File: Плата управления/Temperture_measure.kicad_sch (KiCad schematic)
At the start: 3 parts

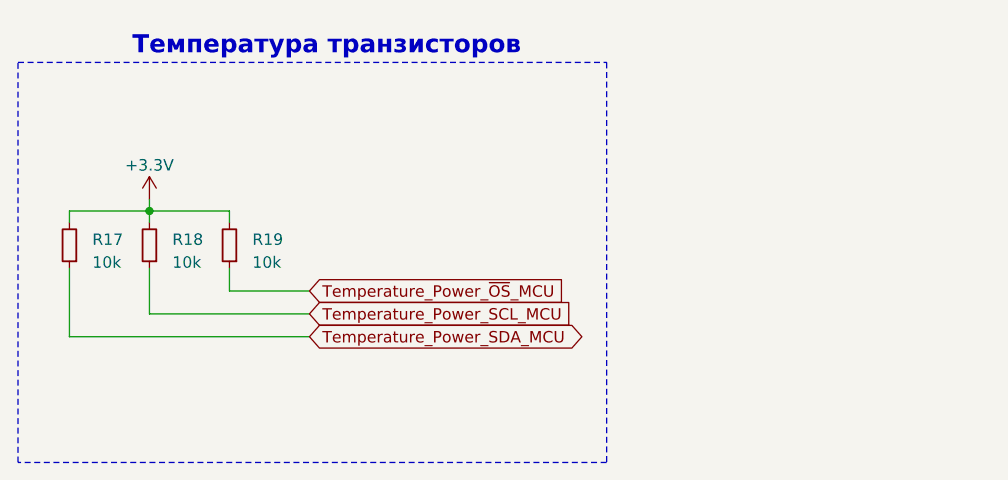
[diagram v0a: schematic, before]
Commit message: Версия под отчёт
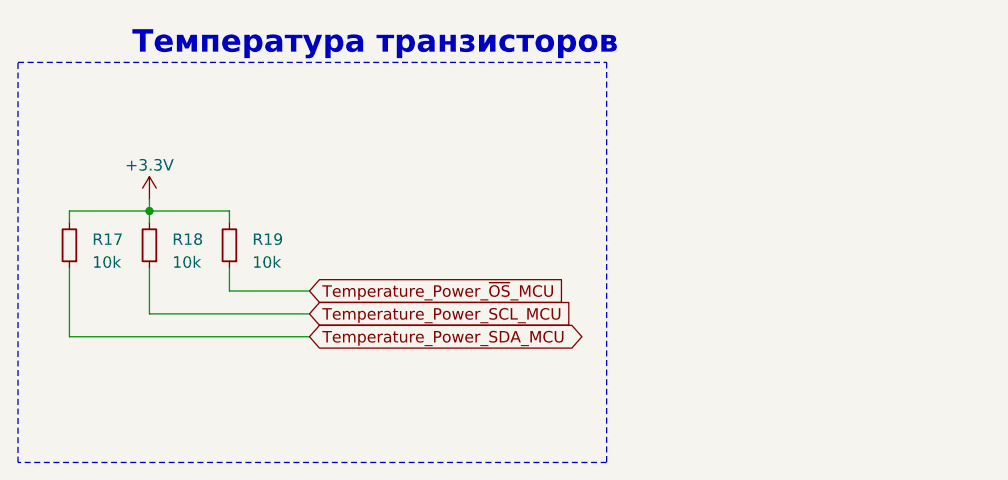
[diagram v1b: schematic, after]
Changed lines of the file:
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@@
   )
   (text "Температура транзисторов" (at 137.795 76.2 0)
-    (effects (font (size 2 2) bold) (justify left bottom))
+    (effects (font (size 2.5 2.5) bold) (justify left bottom))
   )
   (global_label "Temperature_Power_SDA_MCU" (shape bidirectional) (at 157.48 107.315 0) (fields_autoplaced)

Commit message: VER2.0
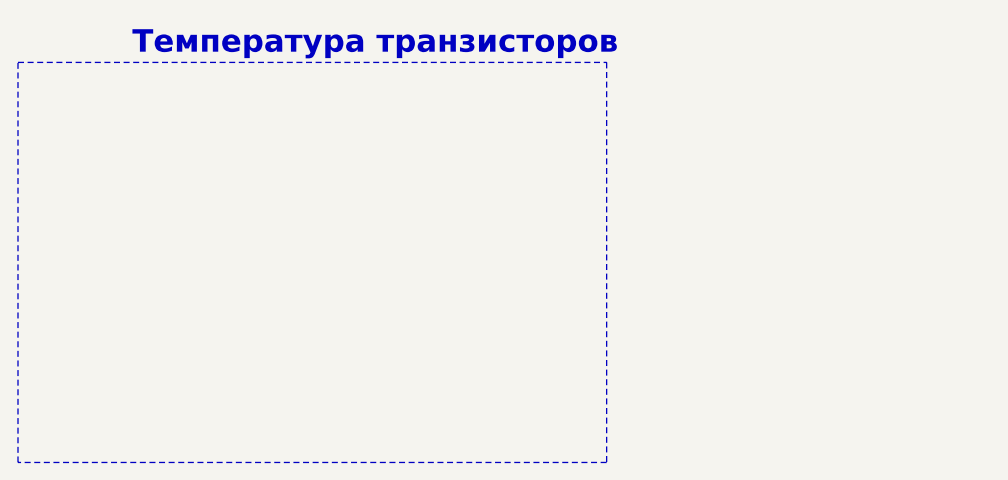
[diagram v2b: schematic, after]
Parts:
- removed R17, R18, R19: 10k, Resistor_SMD:R_0603_1608Metric_Pad0.98x0.95mm_HandSolder, symbol Device:R_Small
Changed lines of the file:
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@@
     (comment 1 "МПСТ.76721.758764.02.Э3.М")
-  )
-  (junction (at 139.7 93.345) (diameter 0) (color 0 0 0 0)
-  )
-  (wire (pts (xy 157.48 107.315) (xy 130.81 107.315))
-    (stroke (width 0) (type default))
-  )
-  (wire (pts (xy 157.48 102.235) (xy 148.59 102.235))
-    (stroke (width 0) (type default))
-  )
-  (wire (pts (xy 139.7 93.345) (xy 139.7 94.615))
-    (stroke (width 0) (type default))
-  )
-  (wire (pts (xy 139.7 92.075) (xy 139.7 93.345))
-    (stroke (width 0) (type default))
-  )
-  (wire (pts (xy 139.7 104.775) (xy 139.7 99.695))
-    (stroke (width 0) (type default))
-  )
-  (wire (pts (xy 148.59 94.615) (xy 148.59 93.345))
-    (stroke (width 0) (type default))
-  )
-  (wire (pts (xy 148.59 102.235) (xy 148.59 99.695))
-    (stroke (width 0) (type default))
-  )
-  (wire (pts (xy 130.81 93.345) (xy 139.7 93.345))
-    (stroke (width 0) (type default))
-  )
-  (wire (pts (xy 139.7 93.345) (xy 148.59 93.345))
-    (stroke (width 0) (type default))
-  )
-  (wire (pts (xy 130.81 94.615) (xy 130.81 93.345))
-    (stroke (width 0) (type default))
-  )
-  (wire (pts (xy 130.81 107.315) (xy 130.81 99.695))
-    (stroke (width 0) (type default))
-  )
-  (wire (pts (xy 157.48 104.775) (xy 139.7 104.775))
-    (stroke (width 0) (type default))
   )
   (rectangle (start 125.095 76.835) (end 190.5 121.285)
@@
     (effects (font (size 2.5 2.5) bold) (justify left bottom))
   )
-  (global_label "Temperature_Power_SDA_MCU" (shape bidirectional) (at 157.48 107.315 0) (fields_autoplaced)
-    (effects (font (size 1.27 1.27)) (justify left))
-    (property "Intersheetrefs" "${INTERSHEET_REFS}" (at 189.3954 107.315 0)
-      (effects (font (size 1.27 1.27)) (justify left) hide)
-    )
-  )
-  (global_label "Temperature_Power_SCL_MCU" (shape input) (at 157.48 104.775 0) (fields_autoplaced)
-    (effects (font (size 1.27 1.27)) (justify left))
-    (property "Intersheetrefs" "${INTERSHEET_REFS}" (at 188.2236 104.775 0)
-      (effects (font (size 1.27 1.27)) (justify left) hide)
-    )
-  )
-  (global_label "Temperature_Power_~{OS}_MCU" (shape input) (at 157.48 102.235 0) (fields_autoplaced)
-    (effects (font (size 1.27 1.27)) (justify left))
-    (property "Intersheetrefs" "${INTERSHEET_REFS}" (at 187.256 102.235 0)
-      (effects (font (size 1.27 1.27)) (justify left) hide)
-    )
-  )
-  (symbol (lib_id "Device:R_Small") (at 148.59 97.155 180) (unit 1)
-    (in_bom yes) (on_board yes) (dnp no) (fields_autoplaced)
-    (property "Reference" "R19" (at 151.13 96.52 0)
-      (effects (font (size 1.27 1.27)) (justify right))
-    )
-    (property "Value" "10k" (at 151.13 99.06 0)
-      (effects (font (size 1.27 1.27)) (justify right))
-    )
-    (property "Footprint" "Resistor_SMD:R_0603_1608Metric_Pad0.98x0.95mm_HandSolder" (at 148.59 97.155 0)
-      (effects (font (size 1.27 1.27)) hide)
-    )
-    (property "Datasheet" "~" (at 148.59 97.155 0)
-      (effects (font (size 1.27 1.27)) hide)
-    )
-    (pin "1")
-    (pin "2")
-    (instances
-      (project "Плата управления"
-        (path "/75f4c67c-bbde-4446-8f82-67797a1b269f/d6b8b9ce-300b-4d22-9d4c-9182eba581b1"
-          (reference "R19") (unit 1)
-        )
-        (path "/75f4c67c-bbde-4446-8f82-67797a1b269f/c91ff3ec-ad20-4326-acd4-2c9dea437172"
-          (reference "R17") (unit 1)
-        )
-      )
-      (project "Силовая плата"
-        (path "/96c6fc92-8ec6-44f7-b0dc-9ad8f1acea09/1efb5faf-bb82-4ac6-a144-d6576b4720aa"
-          (reference "R2") (unit 1)
-        )
-      )
-    )
-  )
-  (symbol (lib_id "power:+3.3V") (at 139.7 92.075 0) (unit 1)
-    (in_bom yes) (on_board yes) (dnp no) (fields_autoplaced)
-    (property "Reference" "#PWR026" (at 139.7 95.885 0)
-      (effects (font (size 1.27 1.27)) hide)
-    )
-    (property "Value" "+3.3V" (at 139.7 88.265 0)
-      (effects (font (size 1.27 1.27)))
-    )
-    (property "Footprint" "" (at 139.7 92.075 0)
-      (effects (font (size 1.27 1.27)) hide)
-    )
-    (property "Datasheet" "" (at 139.7 92.075 0)
-      (effects (font (size 1.27 1.27)) hide)
-    )
-    (pin "1")
-    (instances
-      (project "Плата управления"
-        (path "/75f4c67c-bbde-4446-8f82-67797a1b269f/d6b8b9ce-300b-4d22-9d4c-9182eba581b1"
-          (reference "#PWR026") (unit 1)
-        )
-      )
-    )
-  )
-  (symbol (lib_id "Device:R_Small") (at 130.81 97.155 180) (unit 1)
-    (in_bom yes) (on_board yes) (dnp no) (fields_autoplaced)
-    (property "Reference" "R17" (at 133.35 96.52 0)
-      (effects (font (size 1.27 1.27)) (justify right))
-    )
-    (property "Value" "10k" (at 133.35 99.06 0)
-      (effects (font (size 1.27 1.27)) (justify right))
-    )
-    (property "Footprint" "Resistor_SMD:R_0603_1608Metric_Pad0.98x0.95mm_HandSolder" (at 130.81 97.155 0)
-      (effects (font (size 1.27 1.27)) hide)
-    )
-    (property "Datasheet" "~" (at 130.81 97.155 0)
-      (effects (font (size 1.27 1.27)) hide)
-    )
-    (pin "1")
-    (pin "2")
-    (instances
-      (project "Плата управления"
-        (path "/75f4c67c-bbde-4446-8f82-67797a1b269f/d6b8b9ce-300b-4d22-9d4c-9182eba581b1"
-          (reference "R17") (unit 1)
-        )
-        (path "/75f4c67c-bbde-4446-8f82-67797a1b269f/c91ff3ec-ad20-4326-acd4-2c9dea437172"
-          (reference "R17") (unit 1)
-        )
-      )
-      (project "Силовая плата"
-        (path "/96c6fc92-8ec6-44f7-b0dc-9ad8f1acea09/1efb5faf-bb82-4ac6-a144-d6576b4720aa"
-          (reference "R2") (unit 1)
-        )
-      )
-    )
-  )
-  (symbol (lib_id "Device:R_Small") (at 139.7 97.155 180) (unit 1)
-    (in_bom yes) (on_board yes) (dnp no) (fields_autoplaced)
-    (property "Reference" "R18" (at 142.24 96.52 0)
-      (effects (font (size 1.27 1.27)) (justify right))
-    )
-    (property "Value" "10k" (at 142.24 99.06 0)
-      (effects (font (size 1.27 1.27)) (justify right))
-    )
-    (property "Footprint" "Resistor_SMD:R_0603_1608Metric_Pad0.98x0.95mm_HandSolder" (at 139.7 97.155 0)
-      (effects (font (size 1.27 1.27)) hide)
-    )
-    (property "Datasheet" "~" (at 139.7 97.155 0)
-      (effects (font (size 1.27 1.27)) hide)
-    )
-    (pin "1")
-    (pin "2")
-    (instances
-      (project "Плата управления"
-        (path "/75f4c67c-bbde-4446-8f82-67797a1b269f/d6b8b9ce-300b-4d22-9d4c-9182eba581b1"
-          (reference "R18") (unit 1)
-        )
-        (path "/75f4c67c-bbde-4446-8f82-67797a1b269f/c91ff3ec-ad20-4326-acd4-2c9dea437172"
-          (reference "R17") (unit 1)
-        )
-      )
-      (project "Силовая плата"
-        (path "/96c6fc92-8ec6-44f7-b0dc-9ad8f1acea09/1efb5faf-bb82-4ac6-a144-d6576b4720aa"
-          (reference "R2") (unit 1)
-        )
-      )
-    )
-  )
 )
